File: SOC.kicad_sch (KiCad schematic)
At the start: 10 parts, among them J3 TF01-A, J4 CL24CR492, P1 HRO-TYPE-C-31-M-12, SW2 TS-1157-X-A, SW3 TS-1157-X-A, SW4 TS-1157-X-A, SW5 TS-1157-X-A, SW6 TS-1157-X-A, U12 W25Q128JVSIQ, U13 F1C200S

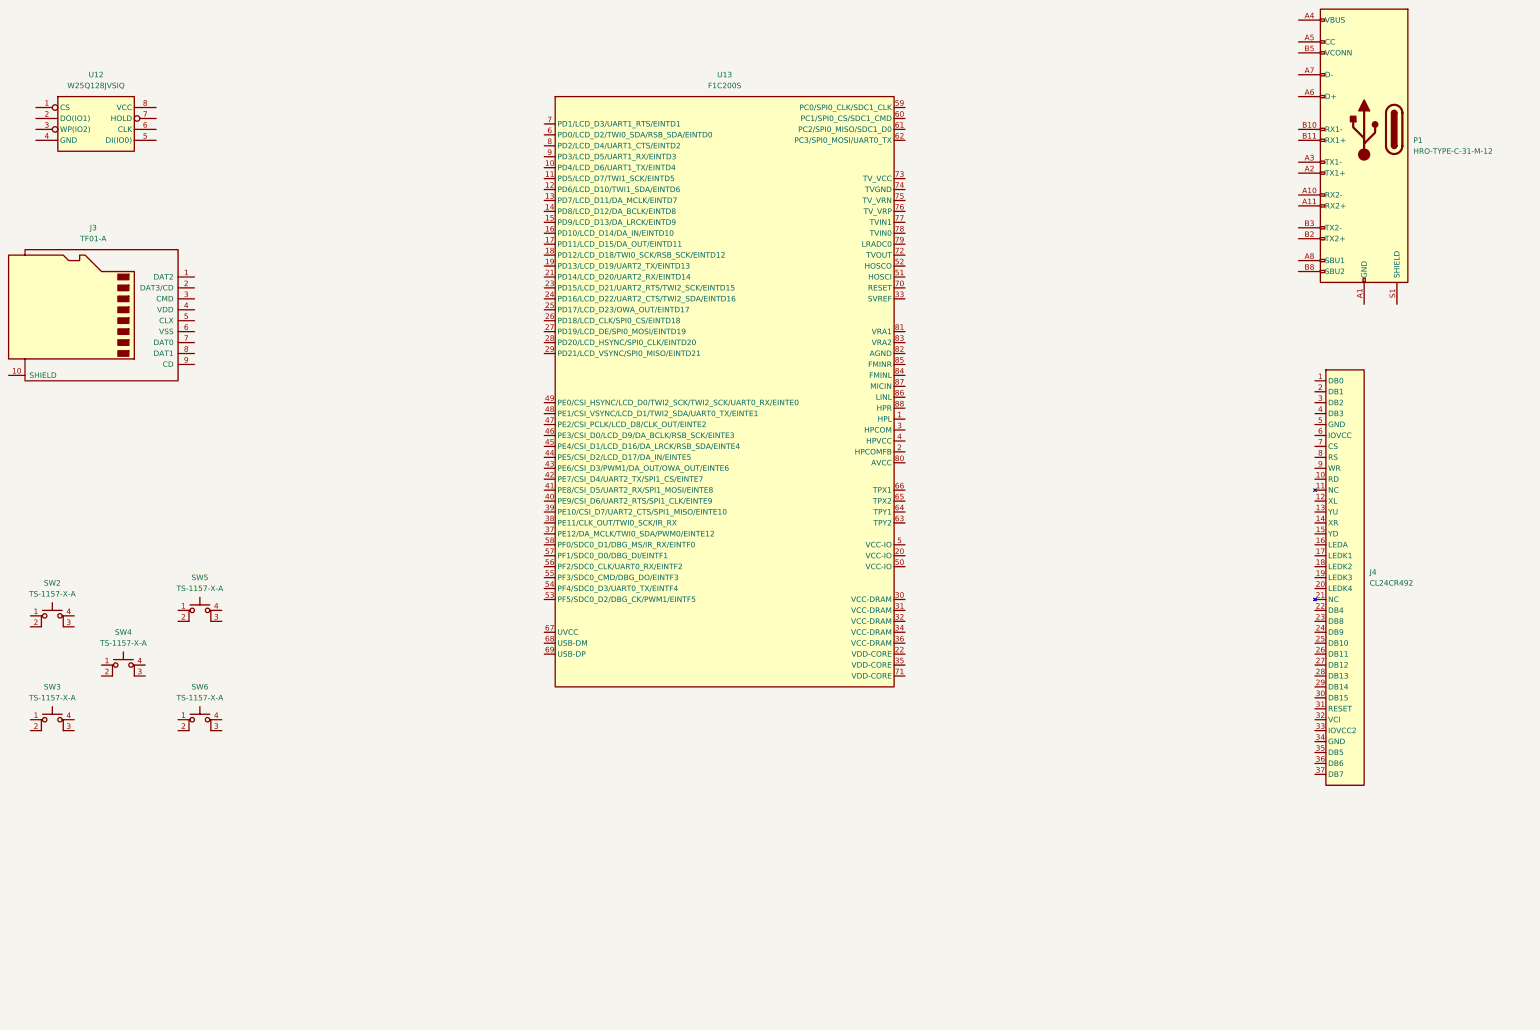
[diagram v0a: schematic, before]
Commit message: dfdfasfasf
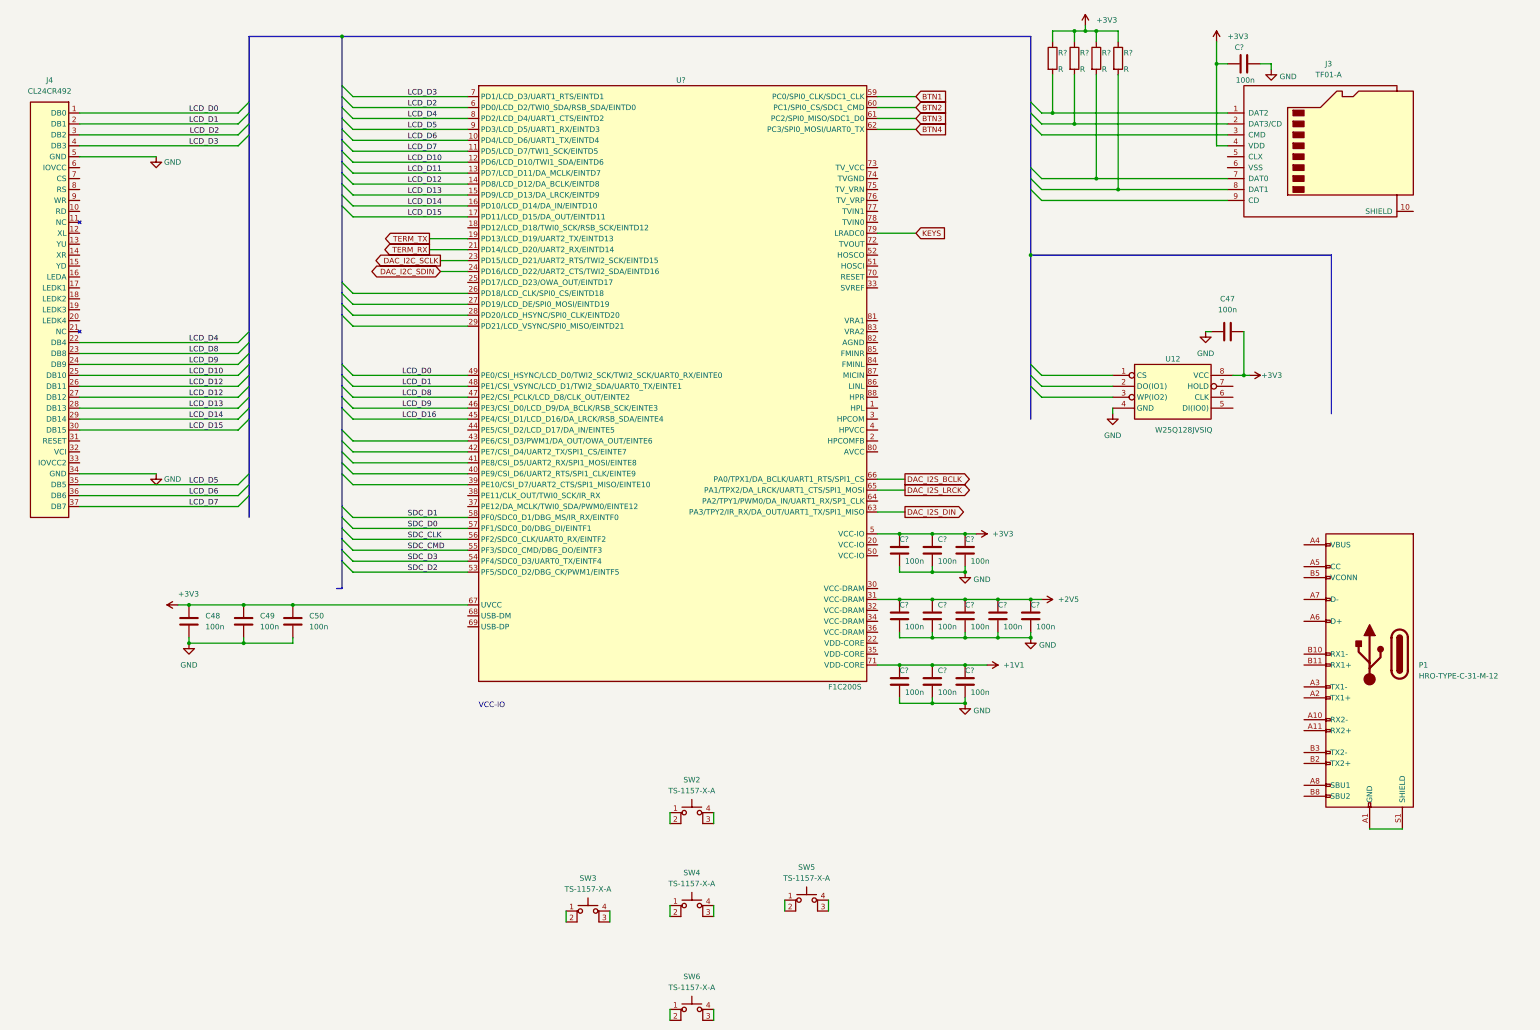
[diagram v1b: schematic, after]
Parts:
- removed U13: F1C200S, rlib_ic:QFN-88_EP_10x10_Pitch0.4mm, symbol rlib_ic:F1C200S
- added C47, C48, C49, C50, C? (x12): 100n, symbol rlib_passive:C
- added R? (x4): R, symbol rlib_passive:R
- added U?: F1C200S, rlib_ic:QFN-88_EP_10x10_Pitch0.4mm, symbol rlib_ic:F1C200S
- U12: footprint Package_SO:SOIC-8_5.23x5.23mm_P1.27mm -> rlib_ic:SOIC-8_5.23x5.23mm_P1.27mm
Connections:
- net at SW3.1: now also SW3.2
- net at SW3.3 (K): now also SW3.4 (A)
- net at SW4.1: now also SW4.2
- net at SW4.3 (K): now also SW4.4 (A)
- net LCD_D0: now reaches J4.1 (DB0)
- net LCD_D0: now also U?.49 (PE0/CSI_HSYNC/LCD_D0/TWI2_SCK/TWI2_SCK/UART0_RX/EINTE0)
- net LCD_D1: now reaches J4.2 (DB1)
- net LCD_D1: now also U?.48 (PE1/CSI_VSYNC/LCD_D1/TWI2_SDA/UART0_TX/EINTE1)
- net LCD_D4: now reaches J4.22 (DB4)
- net LCD_D4: now also U?.8 (PD2/LCD_D4/UART1_CTS/EINTD2)
- net LCD_D8: now reaches J4.23 (DB8)
- net LCD_D8: now also U?.47 (PE2/CSI_PCLK/LCD_D8/CLK_OUT/EINTE2)
- net LCD_D9: now reaches J4.24 (DB9)
- net LCD_D9: now also U?.46 (PE3/CSI_D0/LCD_D9/DA_BCLK/RSB_SCK/EINTE3)
- net LCD_D10: now reaches J4.25 (DB10)
- net LCD_D10: now also U?.12 (PD6/LCD_D10/TWI1_SDA/EINTD6)
- net LCD_D12: now reaches J4.26 (DB11)
- net LCD_D12: now also J4.27 (DB12), U?.14 (PD8/LCD_D12/DA_BCLK/EINTD8)
- net LCD_D13: now reaches J4.28 (DB13)
- net LCD_D13: now also U?.15 (PD9/LCD_D13/DA_LRCK/EINTD9)
- net LCD_D14: now reaches J4.29 (DB14)
- net LCD_D14: now also U?.16 (PD10/LCD_D14/DA_IN/EINTD10)
- net LCD_D2: now reaches J4.3 (DB2)
- net LCD_D2: now also U?.6 (PD0/LCD_D2/TWI0_SDA/RSB_SDA/EINTD0)
- net LCD_D15: now reaches J4.30 (DB15)
- net LCD_D15: now also U?.17 (PD11/LCD_D15/DA_OUT/EINTD11)
- net GND: now reaches J4.34 (GND)
- net GND: now also J4.5 (GND), U12.4 (GND), C47.1, C48.2, C49.2, C50.2, C?.2, C?.2, C?.2, C?.2, C?.2, C?.2, C?.2, C?.2, C?.2, C?.2, C?.2, C?.2
- net LCD_D5: now reaches J4.35 (DB5)
- net LCD_D5: now also U?.9 (PD3/LCD_D5/UART1_RX/EINTD3)
- net LCD_D6: now reaches J4.36 (DB6)
- net LCD_D6: now also U?.10 (PD4/LCD_D6/UART1_TX/EINTD4)
- net LCD_D7: now reaches J4.37 (DB7)
- net LCD_D7: now also U?.11 (PD5/LCD_D7/TWI1_SCK/EINTD5)
- net LCD_D3: now reaches J4.4 (DB3)
- net LCD_D3: now also U?.7 (PD1/LCD_D3/UART1_RTS/EINTD1)
- net at SW2.1: now also SW2.2
- net at SW2.3 (K): now also SW2.4 (A)
- net at SW6.1: now also SW6.2
- net at SW6.3 (K): now also SW6.4 (A)
- net at SW5.1: now also SW5.2
- net at SW5.3 (K): now also SW5.4 (A)
- net at P1.A1 (GND), P1.A12 (GND), P1.B1 (GND)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: now also P1.S1 (SHIELD)
- net +3V3: now reaches U12.8 (VCC)
- net +3V3: now also J3.4 (VDD), C47.2, C48.1, C49.1, C50.1, C?.1, C?.1, C?.1, C?.1, R?.1, R?.1, R?.1, R?.1, U?.5 (VCC-IO), U?.67 (UVCC)
- net at J3.1 (DAT2): now also R?.2
- net at J3.2 (DAT3/CD): now also R?.2
- net at J3.7 (DAT0): now also R?.2
- net at J3.8 (DAT1): now also R?.2
- new net +1V1: C?.1, C?.1, C?.1, U?.71 (VDD-CORE)
- new net +2V5: C?.1, C?.1, C?.1, C?.1, C?.1, U?.31 (VCC-DRAM)
- new net BTN1: U?.59 (PC0/SPI0_CLK/SDC1_CLK)
- new net BTN2: U?.60 (PC1/SPI0_CS/SDC1_CMD)
- new net BTN3: U?.61 (PC2/SPI0_MISO/SDC1_D0)
- new net BTN4: U?.62 (PC3/SPI0_MOSI/UART0_TX)
- new net DAC_I2C_SCLK: U?.23 (PD15/LCD_D21/UART2_RTS/TWI2_SCK/EINTD15)
- new net DAC_I2C_SDIN: U?.24 (PD16/LCD_D22/UART2_CTS/TWI2_SDA/EINTD16)
- new net DAC_I2S_BCLK: U?.66 (PA0/TPX1/DA_BCLK/UART1_RTS/SPI1_CS)
- new net DAC_I2S_DIN: U?.63 (PA3/TPY2/IR_RX/DA_OUT/UART1_TX/SPI1_MISO)
- new net DAC_I2S_LRCK: U?.65 (PA1/TPX2/DA_LRCK/UART1_CTS/SPI1_MOSI)
- new net KEYS: U?.79 (LRADC0)
- new net LCD_D11: U?.13 (PD7/LCD_D11/DA_MCLK/EINTD7)
- new net LCD_D16: U?.45 (PE4/CSI_D1/LCD_D16/DA_LRCK/RSB_SDA/EINTE4)
- new net SDC_CLK: U?.56 (PF2/SDC0_CLK/UART0_RX/EINTF2)
- new net SDC_CMD: U?.55 (PF3/SDC0_CMD/DBG_DO/EINTF3)
- new net SDC_D0: U?.57 (PF1/SDC0_D0/DBG_DI/EINTF1)
- new net SDC_D1: U?.58 (PF0/SDC0_D1/DBG_MS/IR_RX/EINTF0)
- new net SDC_D2: U?.53 (PF5/SDC0_D2/DBG_CK/PWM1/EINTF5)
- new net SDC_D3: U?.54 (PF4/SDC0_D3/UART0_TX/EINTF4)
- new net TERM_RX: U?.21 (PD14/LCD_D20/UART2_RX/EINTD14)
- new net TERM_TX: U?.19 (PD13/LCD_D19/UART2_TX/EINTD13)
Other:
- note added: "VCC-IO"
- moved on the sheet: J3, J4, P1, SW2, SW3, SW4, SW5, SW6, U12
